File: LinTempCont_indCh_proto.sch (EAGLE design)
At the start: 26 parts

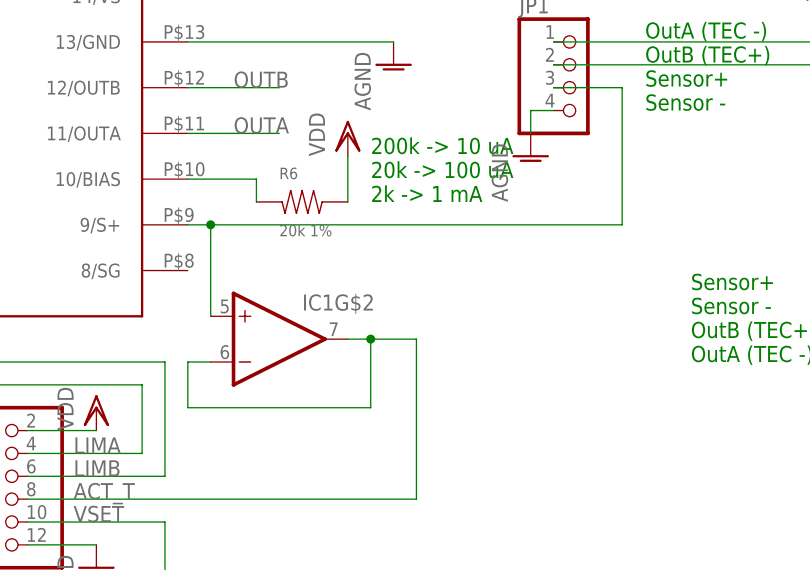
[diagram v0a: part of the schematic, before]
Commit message: Board/Schematic updates and tweaks
Incorporate suggestions from Neal and Alessandro
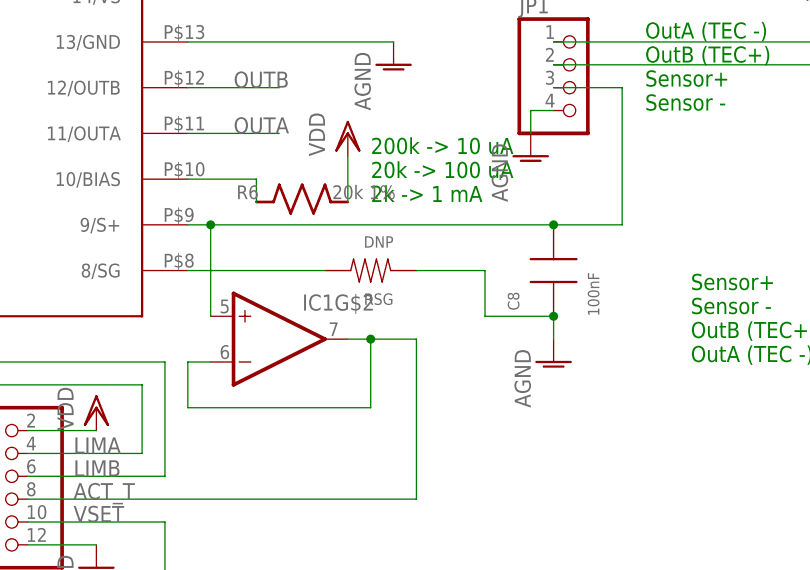
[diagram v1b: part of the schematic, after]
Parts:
- added C8: 100nF, rlc-jqi:CAP0603
- added RSG: DNP, rlc-jqi:RES0603
- R6: device rlc-jqi:RES0603 -> jqi_passives:R_SMDR0805
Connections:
- new net N$6: RSG.P$2, U1.8/SG
- net AGND: now also C8.P$1, RSG.P$1
- net N$2: now also C8.P$2
- net N$4: now also R6.1; no longer R6.P$1
- net VDD: now also R6.2; no longer R6.P$2
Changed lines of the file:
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@@
 <part name="C3" library="rlc-jqi" deviceset="CAP" device="0603" value="10uF"/>
 <part name="VDD1" library="supply1" deviceset="VDD" device=""/>
-<part name="R6" library="rlc-jqi" deviceset="RES" device="0603" value="20k 1%"/>
+<part name="R6" library="jqi_passives" deviceset="R_SMD" device="R0805" value="20k 1%"/>
 <part name="VDD2" library="supply1" deviceset="VDD" device=""/>
 <part name="AGND5" library="supply1" deviceset="AGND" device=""/>
@@
 <part name="VDD3" library="supply1" deviceset="VDD" device=""/>
 <part name="VDD4" library="supply1" deviceset="VDD" device=""/>
+<part name="C8" library="rlc-jqi" deviceset="CAP" device="0603" value="100nF"/>
+<part name="AGND1" library="supply1" deviceset="AGND" device=""/>
+<part name="RSG" library="rlc-jqi" deviceset="RES" device="0603" value="DNP"/>
 </parts>
 <sheets>
@@
 <instance part="VDD3" gate="G$1" x="-5.08" y="-45.72"/>
 <instance part="VDD4" gate="G$1" x="40.64" y="-33.02"/>
+<instance part="C8" gate="G$1" x="91.44" y="-17.78" rot="R90"/>
+<instance part="AGND1" gate="VR1" x="91.44" y="-27.94"/>
+<instance part="RSG" gate="G$1" x="71.12" y="-17.78" rot="R180"/>
 </instances>
 <busses>
@@
 <pinref part="AGND6" gate="VR1" pin="AGND"/>
 </segment>
+<segment>
+<pinref part="C8" gate="G$1" pin="P$1"/>
+<pinref part="AGND1" gate="VR1" pin="AGND"/>
+<wire x1="91.44" y1="-25.4" x2="91.44" y2="-22.86" width="0.1524" layer="91"/>
+<pinref part="RSG" gate="G$1" pin="P$1"/>
+<wire x1="76.2" y1="-17.78" x2="83.82" y2="-17.78" width="0.1524" layer="91"/>
+<wire x1="83.82" y1="-17.78" x2="83.82" y2="-22.86" width="0.1524" layer="91"/>
+<wire x1="83.82" y1="-22.86" x2="91.44" y2="-22.86" width="0.1524" layer="91"/>
+<junction x="91.44" y="-22.86"/>
+</segment>
 </net>
 <net name="VDD" class="0">
@@
 </segment>
 <segment>
-<pinref part="R6" gate="G$1" pin="P$2"/>
+<pinref part="R6" gate="G$1" pin="2"/>
 <pinref part="VDD2" gate="G$1" pin="VDD"/>
 <wire x1="68.58" y1="-10.16" x2="68.58" y2="-5.08" width="0.1524" layer="91"/>
@@
 <segment>
 <pinref part="U1" gate="G$1" pin="9/S+"/>
-<wire x1="99.06" y1="-12.7" x2="53.34" y2="-12.7" width="0.1524" layer="91"/>
+<wire x1="99.06" y1="-12.7" x2="91.44" y2="-12.7" width="0.1524" layer="91"/>
 <pinref part="IC1" gate="G$2" pin="+IN"/>
+<wire x1="91.44" y1="-12.7" x2="53.34" y2="-12.7" width="0.1524" layer="91"/>
 <wire x1="53.34" y1="-12.7" x2="50.8" y2="-12.7" width="0.1524" layer="91"/>
 <wire x1="53.34" y1="-22.86" x2="53.34" y2="-12.7" width="0.1524" layer="91"/>
@@
 <pinref part="JP1" gate="A" pin="3"/>
 <junction x="53.34" y="-12.7"/>
+<pinref part="C8" gate="G$1" pin="P$2"/>
+<junction x="91.44" y="-12.7"/>
 </segment>
 </net>
@@
 <net name="N$4" class="0">
 <segment>
-<pinref part="R6" gate="G$1" pin="P$1"/>
+<pinref part="R6" gate="G$1" pin="1"/>
 <wire x1="58.42" y1="-10.16" x2="58.42" y2="-7.62" width="0.1524" layer="91"/>
 <pinref part="U1" gate="G$1" pin="10/BIAS"/>
@@
 </segment>
 </net>
+<net name="N$6" class="0">
+<segment>
+<pinref part="U1" gate="G$1" pin="8/SG"/>
+<pinref part="RSG" gate="G$1" pin="P$2"/>
+<wire x1="66.04" y1="-17.78" x2="50.8" y2="-17.78" width="0.1524" layer="91"/>
+</segment>
+</net>
